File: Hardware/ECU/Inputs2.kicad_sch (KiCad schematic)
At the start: 9 parts, among them Q2 Q_DUAL_NMOS_S1G1D2S2G2D1, U14 LMV324LIDT

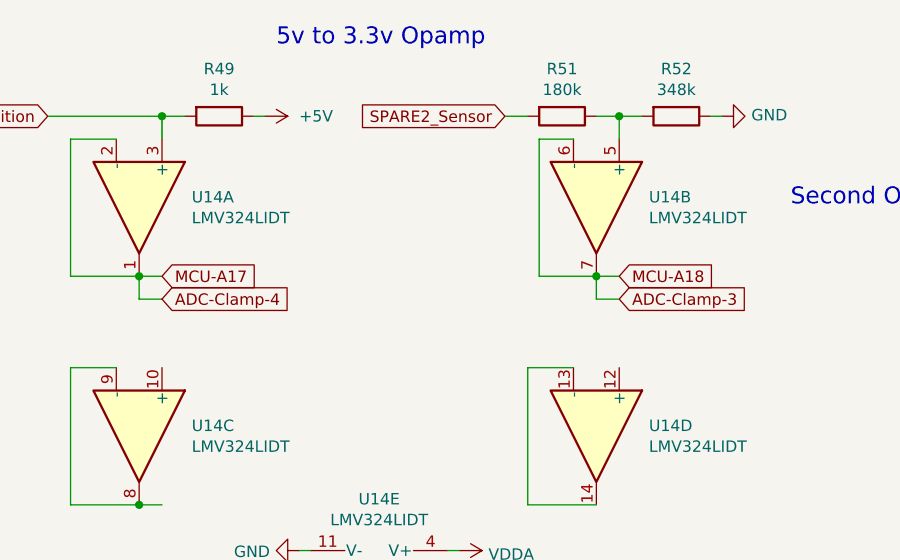
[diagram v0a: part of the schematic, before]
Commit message: deleted:    Hardware/ECU/ECU-backups/ECU-2025-05-27_235240.zip 	deleted:    Hardware/ECU/ECU-backups/ECU-2025-05-28_135321.zip 	deleted:    Hardware/ECU/ECU-backups/ECU-2025-05-28_140049.zip 	deleted:    Hardware/ECU/ECU-backups/ECU-2025-05-28_141416.zip 	deleted:    Hardware/ECU/ECU-backups/ECU-2025-05-28_154718.zip 	deleted:    Hardware/ECU/ECU-backups/ECU-2025-06-18_111329.zip 	new file:   Hardware/ECU/ECU-backups/ECU-2025-08-26_154141.zip 	new file:   Hardware/ECU/ECU-backups/ECU-2025-08-29_143817.zip 	new file:   Hardware/ECU/ECU-backups/ECU-2025-09-19_081818.zip 	new file:   Hardware/ECU/ECU-backups/ECU-2026-01-19_151411.zip 	new file:   Hardware/ECU/ECU-backups/ECU-2026-01-19_152057.zip 	new file:   Hardware/ECU/ECU-backups/ECU-2026-01-19_154705.zip 	modified:   Hardware/ECU/ECU.kicad_pcb 	modified:   Hardware/ECU/ECU.kicad_prl 	modified:   Hardware/ECU/ECU.kicad_sch 	modified:   Hardware/ECU/Inputs.kicad_sch 	modified:   Hardware/ECU/Inputs2.kicad_sch 	renamed:    Hardware/ECU/output/PCB.pdf -> Hardware/ECU/output/PCB-R9.3.pdf 	renamed:    Hardware/ECU/output/Schematics.pdf -> Hardware/ECU/output/Schematics-R0.3.pdf 	new file:   Hardware/ECU/output/Schematics-R1.pdf 	deleted:    Hardware/ECU/output/cut files/ECU-B_Cu.jpg 	modified:   speeduino (modified content)
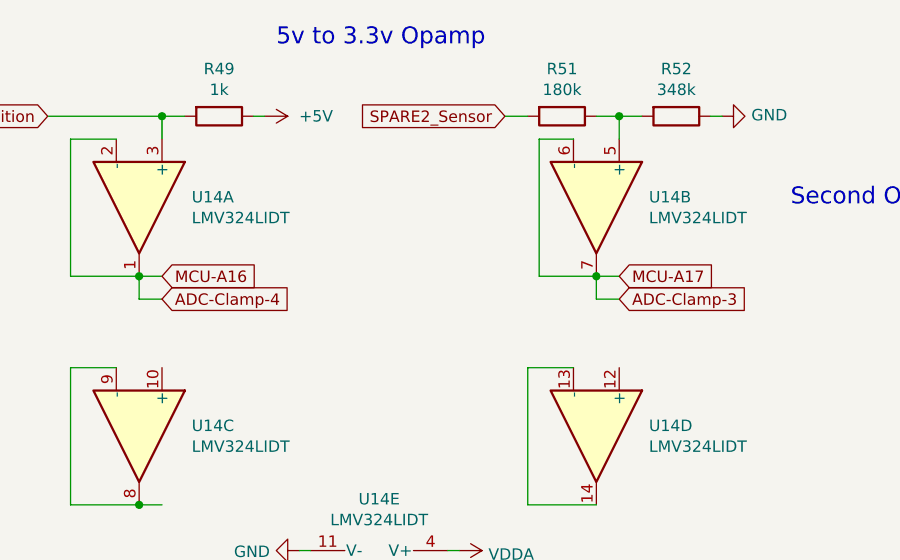
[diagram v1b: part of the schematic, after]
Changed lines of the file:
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@@
 		)
 	)
-	(global_label "MCU-A17"
+	(global_label "MCU-A16"
 		(shape input)
 		(at 118.11 67.31 0)
@@
 		)
 		(property "Intersheetrefs" "${INTERSHEET_REFS}"
-			(at 129.4935 67.31 0)
+			(at 130.2271 67.31 0)
 			(effects
 				(font
@@
 		)
 	)
-	(global_label "MCU-A18"
+	(global_label "MCU-A17"
 		(shape input)
 		(at 168.91 67.31 0)
@@
 		)
 		(property "Intersheetrefs" "${INTERSHEET_REFS}"
-			(at 180.2935 67.31 0)
+			(at 181.0271 67.31 0)
 			(effects
 				(font
